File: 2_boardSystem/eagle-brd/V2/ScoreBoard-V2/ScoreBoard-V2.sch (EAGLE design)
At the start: 42 parts, among them M1 VNH5019, M2 VNH5019, M3 VNH5019, M4 VNH5019, M5 VNH5019, M6 VNH5019, U1 TXB0108PWR

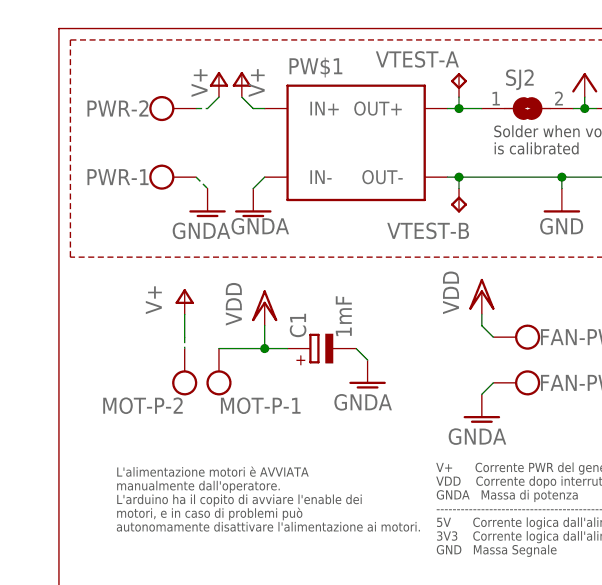
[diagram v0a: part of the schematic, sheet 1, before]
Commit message: board v2 work in progress
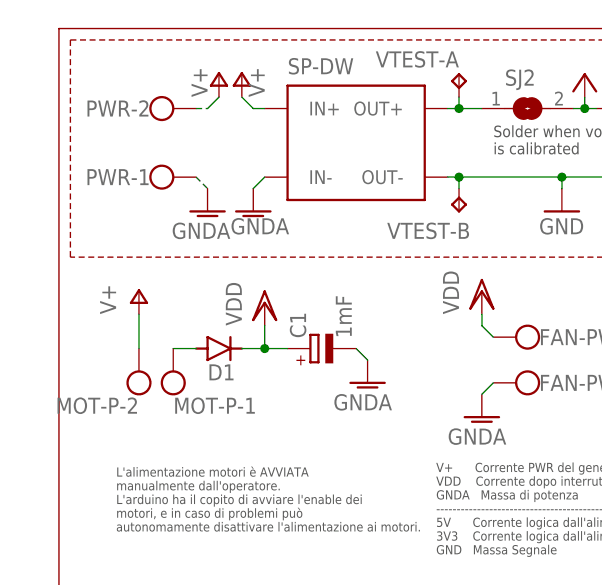
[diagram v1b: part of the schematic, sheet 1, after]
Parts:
- added D1: ES2D, diode:ES2D
- renumbered PW$1 to SP-DW
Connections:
- new net N$2: D1.A, MOT-P-1.KL
- net VDD: now also D1.C; no longer MOT-P-1.KL
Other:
- moved on the sheet: MOT-P-1, MOT-P-2
